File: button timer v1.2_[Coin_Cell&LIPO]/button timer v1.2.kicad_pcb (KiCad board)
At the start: 2 copper layers, 21 x 51.6 mm, 27 parts, among them J1 Conn_01x05_Female, SW1 SW_Push, SW2 SW_Push, U1 TPS61097A, U2 AP2112K-3.3, U3 TPL5111, X1 ESP-12E

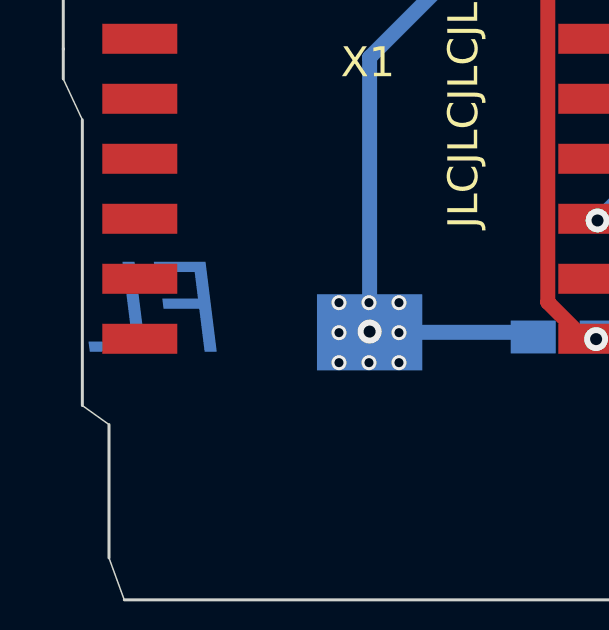
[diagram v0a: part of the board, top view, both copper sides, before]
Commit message: 23.02 00:40
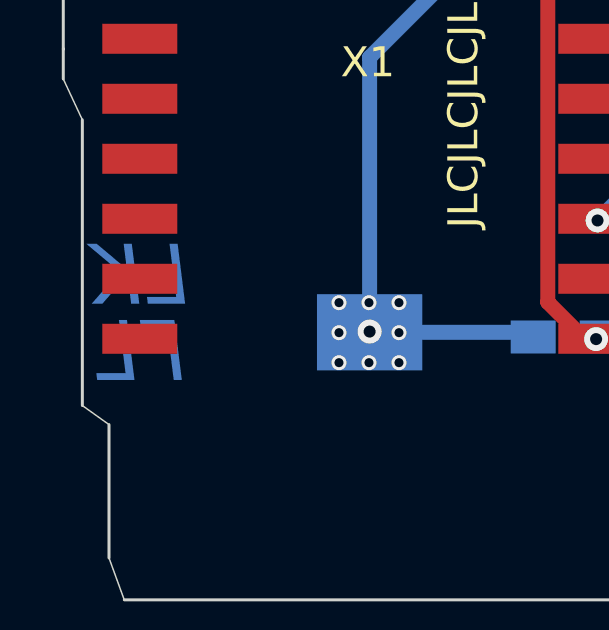
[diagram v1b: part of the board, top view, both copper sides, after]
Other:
- board text added: "LK"
